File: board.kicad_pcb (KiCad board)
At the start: 2 copper layers, 26.9 x 29 mm, 16 parts, among them J1 PMW3360, J2 MCU, J3 Mounting_Hole, J4 Mounting_Hole, J5 Mounting_Hole, J6 Mounting_Hole, U1 TLV70019_SOT23-5

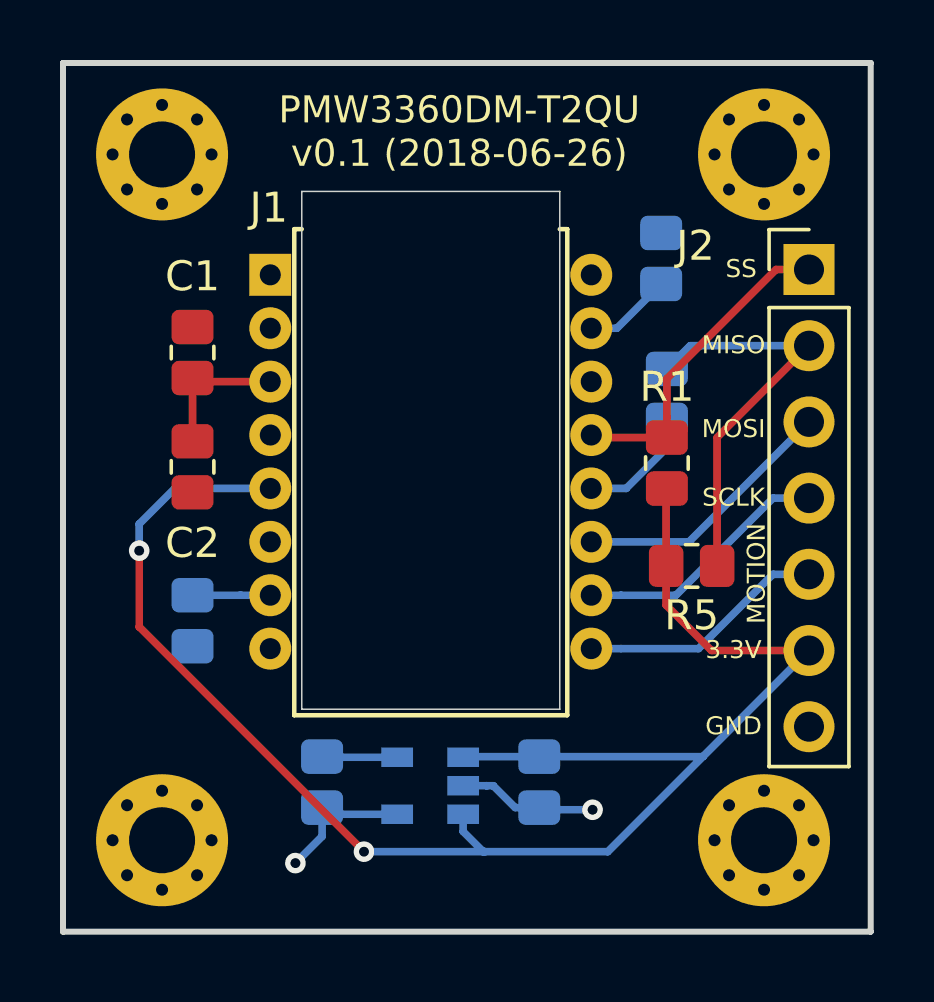
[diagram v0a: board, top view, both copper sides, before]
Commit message: Release 1.0.0
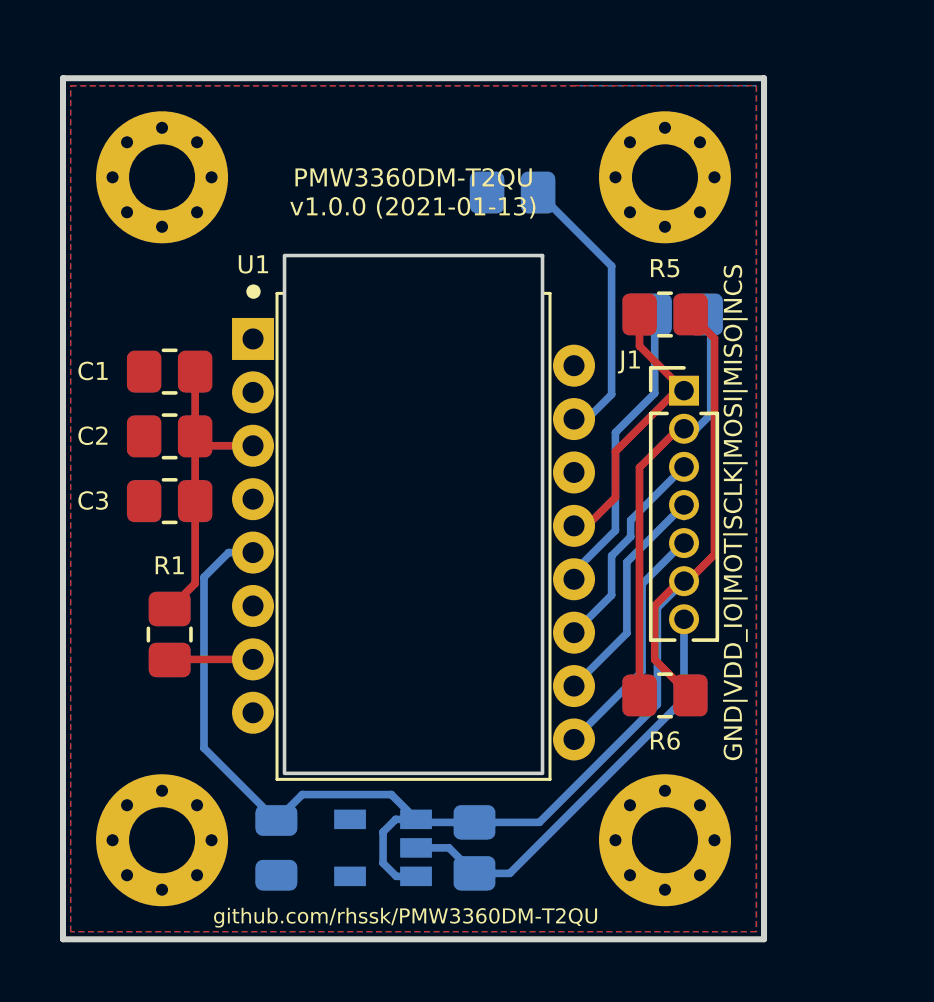
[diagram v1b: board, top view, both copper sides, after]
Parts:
- removed J2: MCU, Connector_PinHeader_2.54mm:PinHeader_1x07_P2.54mm_Vertical
- removed J3, J4, J5, J6: Mounting_Hole, MountingHole:MountingHole_2.2mm_M2_Pad_Via
- added H1: MountingHole, MountingHole:MountingHole_2.2mm_M2_Pad_Via, F.Cu at (119.4, 50.3)
- added H2: MountingHole, MountingHole:MountingHole_2.2mm_M2_Pad_Via, F.Cu at (136.1, 50.3)
- added H3: MountingHole, MountingHole:MountingHole_2.2mm_M2_Pad_Via, F.Cu at (119.4, 72.4)
- added H4: MountingHole, MountingHole:MountingHole_2.2mm_M2_Pad_Via, F.Cu at (136.1, 72.4)
- added R4: NL, Resistor_SMD:R_0805_2012Metric, B.Cu at (123.2, 72.6)
- added U2: TLV70019_SOT23-5, Package_TO_SOT_SMD:SOT-23-5, B.Cu at (126.7, 72.6)
- C1: renamed from C4; value 1uF -> 0.1uF; moved to F.Cu
- C2: value 0.1uF -> 1uF
- C3: renamed from C1; value 4.7uF/10V -> 4.7uF
- J1: value PMW3360 -> MCU; footprint Pixart:PMW3360DM-T2QU -> Connector_PinHeader_1.27mm:PinHeader_1x07_P1.27mm_Vertical
- R1: renamed from R3; moved to F.Cu
- U1: value TLV70019_SOT23-5 -> PMW3360DM-T2QU; footprint Package_TO_SOT_SMD:SOT-23-5 -> Pixart:PMW3360DM-T2QU; moved to F.Cu
- moved J1 16.1 mm to (136.8, 57.4)
- moved C1 14.6 mm to (119.6, 56.8), turned to 0 degrees
- moved U1 9.25 mm to (127.8, 61.3), turned to -90 degrees
- moved R2 5.42 mm to (131.1, 50.8), turned to 0 degrees
- moved C3 5.01 mm to (119.6, 61.1), turned to 180 degrees
- moved R5 4.95 mm to (136.1, 54.9), turned to 0 degrees
- moved R6 4.41 mm to (136.1, 67.6), turned to 0 degrees
- moved C4 3.08 mm to (129.8, 72.6)
- moved R3 2.70 mm to (136.7, 54.9), turned to 0 degrees
- moved C2 1.27 mm to (119.6, 58.9), turned to 180 degrees
- moved R1 0.89 mm to (119.6, 65.5), turned to -90 degrees
- renumbered C3 to C4, R4 to R3, R1 to R5, R5 to R6
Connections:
- C1 pad 1: 1.9V -> GND
- C1 pad 2: GND -> VDD
- C2 pad 1: Net-(C1-Pad1) -> VDD
- C3 pad 1: Net-(C1-Pad1) -> VDD
- C4 pad 1: +3V3 -> VDD_IO
- J1 pad 1: Net-(J1-Pad1) -> /NCS
- J1 pad 2: Net-(J1-Pad2) -> /MISO
- J1 pad 3: Net-(C1-Pad1) -> /MOSI
- J1 pad 4: 1.9V -> /SCLK
- J1 pad 5: +3V3 -> /MOTION
- J1 pad 6: Net-(J1-Pad6) -> VDD_IO
- J1 pad 7: /RESET -> GND
- R1 pad 1: 1.9V -> VDD
- R1 pad 2: /RESET -> Net-(R1-Pad2)
- R2 pad 1: /LED_P -> VDD
- R2 pad 2: 1.9V -> Net-(R2-Pad2)
- R3 pad 1: Net-(J1-Pad12) -> Net-(R3-Pad1)
- R5 pad 1: /SS -> /NCS
- R5 pad 2: +3V3 -> VDD_IO
- R6 pad 2: +3V3 -> VDD_IO
- U1 pad 1: +3V3 -> no_connect_12
- U1 pad 2: GND -> no_connect_13
- U1 pad 3: +3V3 -> VDD
- U1 pad 4: GND -> VDD
- U1 pad 5: 1.9V -> VDD_IO
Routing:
- net +3V3: track 55.6 -> 0.00 mm, vias 2 -> 0
- net VDD_IO: track 0.00 -> 48.6 mm
- net /SS: track 10.8 -> 0.00 mm
- net VDD: track 0.00 -> 10.3 mm
- net Net-(R3-Pad1): track 0.00 -> 9.99 mm
- net /NCS: track 0.00 -> 9.58 mm
- net Net-(R2-Pad2): track 0.00 -> 9.34 mm
- net GND: track 9.43 -> 14.4 mm, vias 2 -> 0
- net Net-(C1-Pad1): track 4.75 -> 0.00 mm
- net Net-(J1-Pad12): track 4.01 -> 0.00 mm
- net /LED_P: track 2.94 -> 0.00 mm
- net Net-(R1-Pad2): track 0.00 -> 2.79 mm
- net /RESET: track 2.59 -> 0.00 mm
- net 1.9V: track 2.51 -> 0.00 mm
- net /MOSI: track 8.91 -> 7.70 mm
- added copper zone on B.Cu, net VDD
- removed copper zone on B.Cu, net 1.9V
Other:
- board size 26.9 x 29 mm -> 23.4 x 28.7 mm
- net class Default removed
- board text added: "GND|VDD_IO|MOT|SCLK|MOSI|MISO|NCS"
- board text added: "PMW3360DM-T2QU v1.0.0 (2021-01-13)"
- board text added: "github.com/rhssk/PMW3360DM-T2QU"
- board text removed: "3.3V"
- board text removed: "GND"
- board text removed: "MISO"
- board text removed: "MOSI"
- board text removed: "MOTION"
- board text removed: "PMW3360DM-T2QU v0.1 (2018-06-26)"
- board text removed: "SCLK"
- board text removed: "SS"
